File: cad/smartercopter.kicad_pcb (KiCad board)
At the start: 2 copper layers, 37.7 x 16.8 mm, 74 parts, among them P1 CONN_5, P2 CONN_01X01, P3 CONN_01X01, P4 CONN_2, P5 CONN_01X01, P6 CONN_01X01, P7 CONN_01X01, Q1 SiA910EDJ, SW1 SW_PUSH_4, U1 CC2541, U2 MPU-9250, U3 TPS73001, U4 TPS73001, U5 DRV8837, X1 32Mhz

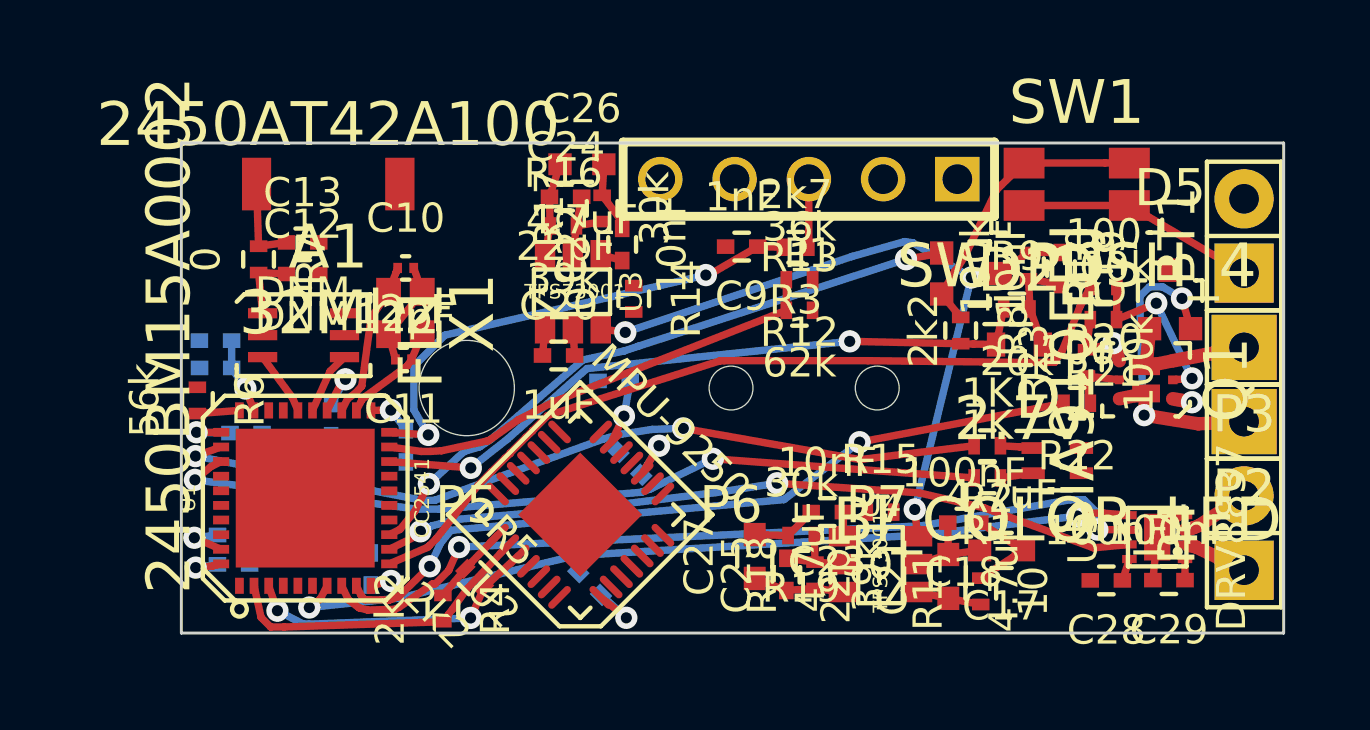
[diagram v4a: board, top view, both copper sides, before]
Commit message: more routing
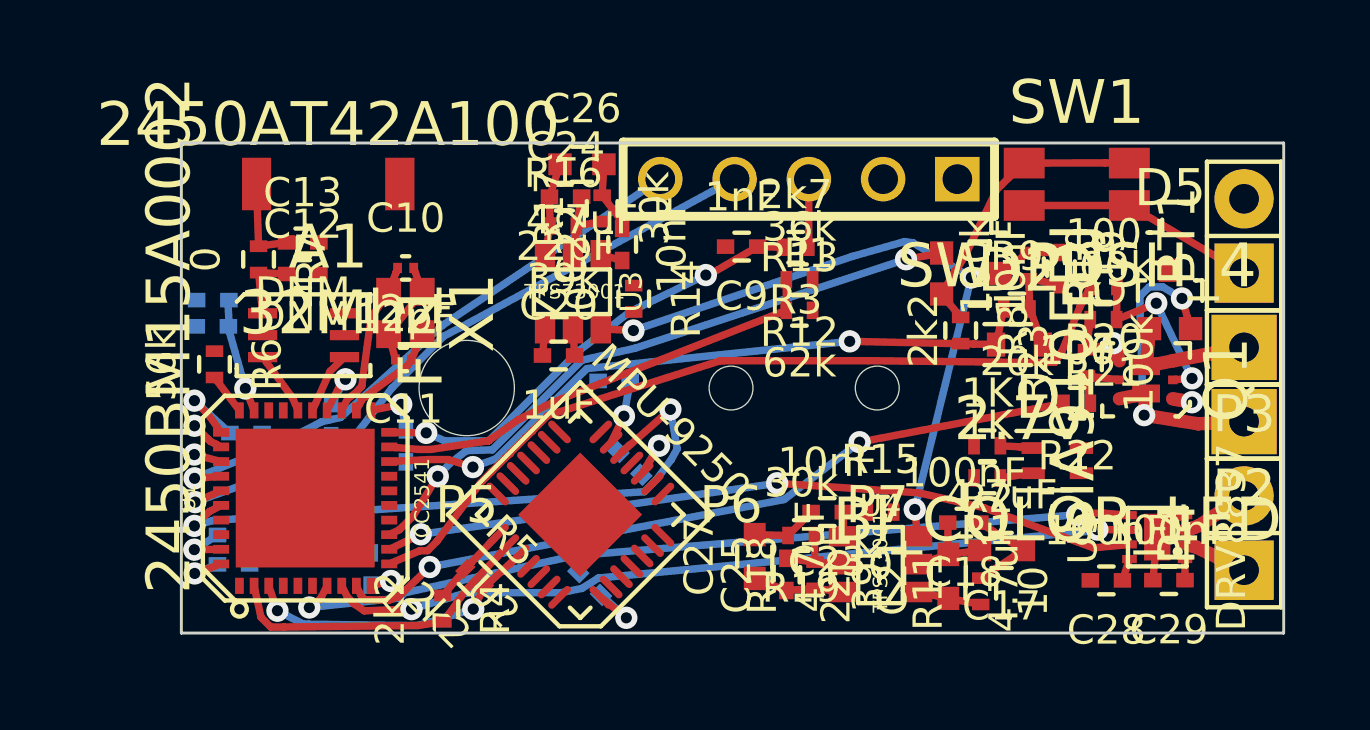
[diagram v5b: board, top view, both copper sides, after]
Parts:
- moved C6 1.43 mm to (52.4, 110.8)
- moved C7 1.39 mm to (52.4, 109.9)
- moved R6 1.36 mm to (52.4, 112.1)
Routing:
- net /LED1: track 28.1 -> 0.95 mm, vias 2 -> 1
- net /LED2: track 28.2 -> 1.18 mm, vias 2 -> 1
- net /DD: track 0.00 -> 22.8 mm, vias 0 -> 1
- net /sensors/INT: track 0.00 -> 22.1 mm, vias 0 -> 2
- net /DC: track 0.00 -> 20.0 mm, vias 0 -> 1
- net VCCA: track 18.7 -> 21.6 mm
- net Net-(C9-Pad1): track 17.4 -> 15.8 mm
- net /motor/PH: track 29.1 -> 27.6 mm
- net /motor/LOW_ROTOR: track 26.5 -> 25.9 mm
